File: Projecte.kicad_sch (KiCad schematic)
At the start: 52 parts, among them J1 Conn_motor, J2 Conn_01x04_Pin, K1 A161CS12VDC.64, Q1 IRLZ34N, Q3 IRLZ34N, Q4 IRLZ34N, Q5 IRLZ34N, Q6 IRLZ34N, Q7 IRLZ34N, U1 PIC18F448-IP, U2 LM358, U3 R-786.5-0.5, U4 MCP2551-I-P, U5 AMS1117-3.3, U6 TXB0108PW, U7 LM7805_TO220, U8 MMC5883MA, Y1 Crystal

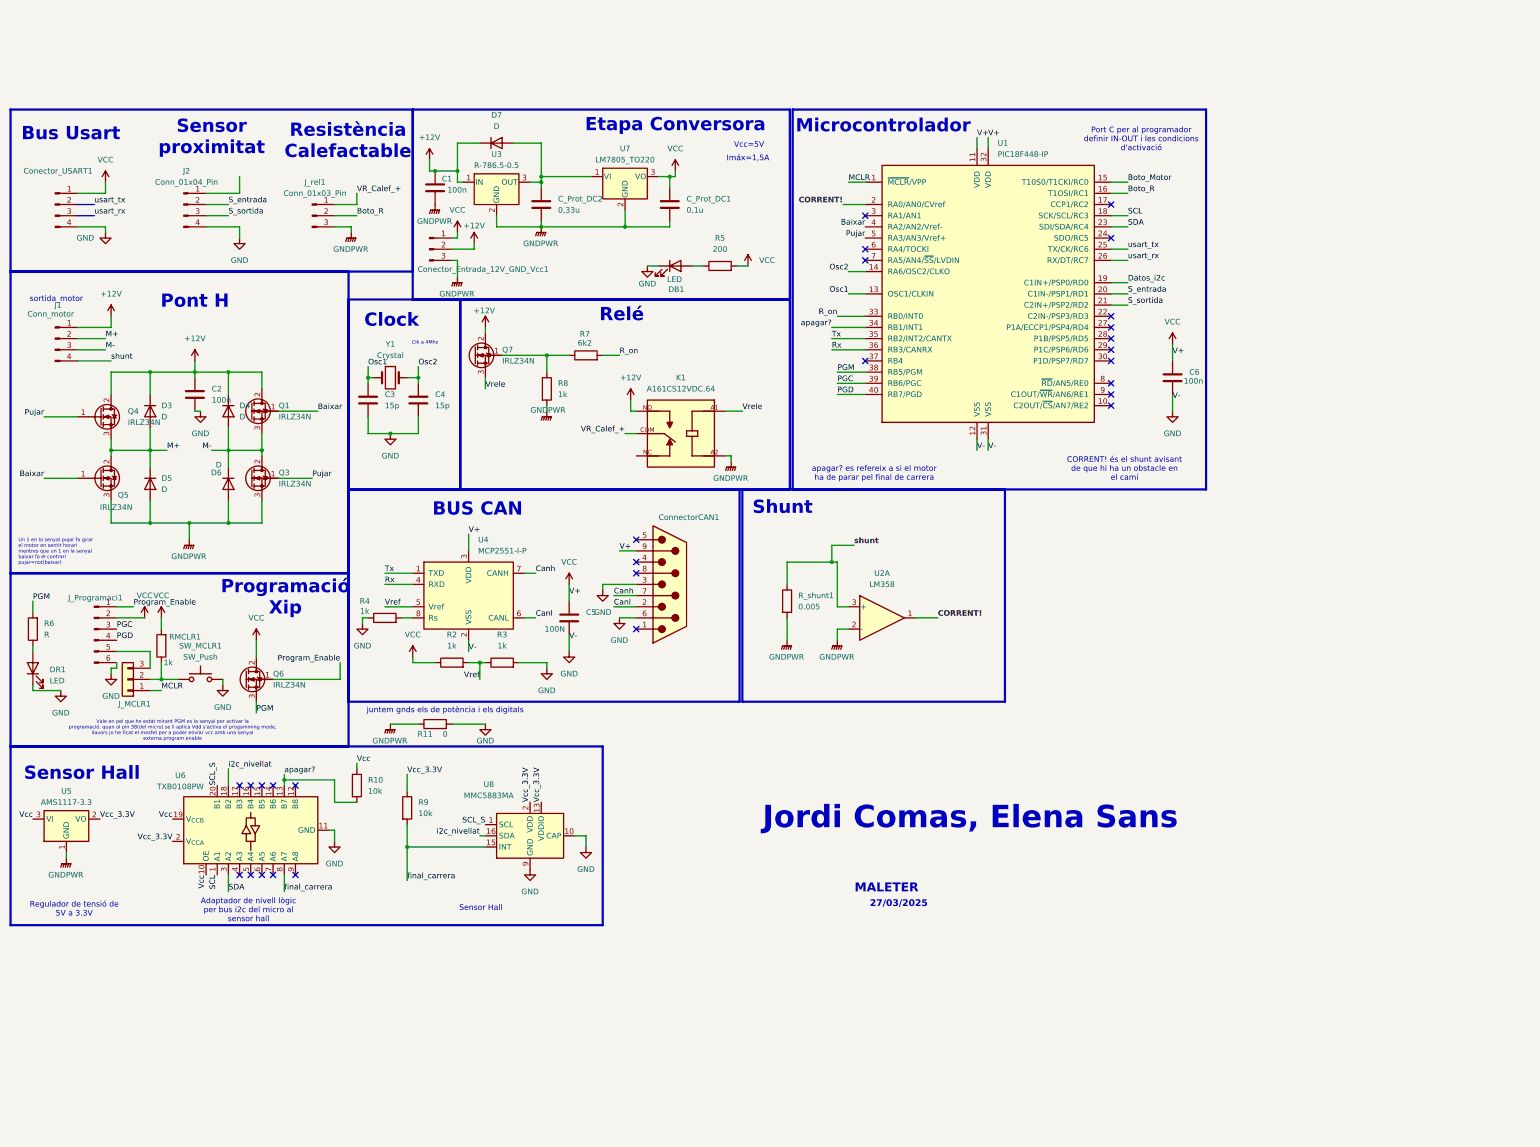
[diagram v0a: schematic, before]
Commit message: Sch_Post_Show
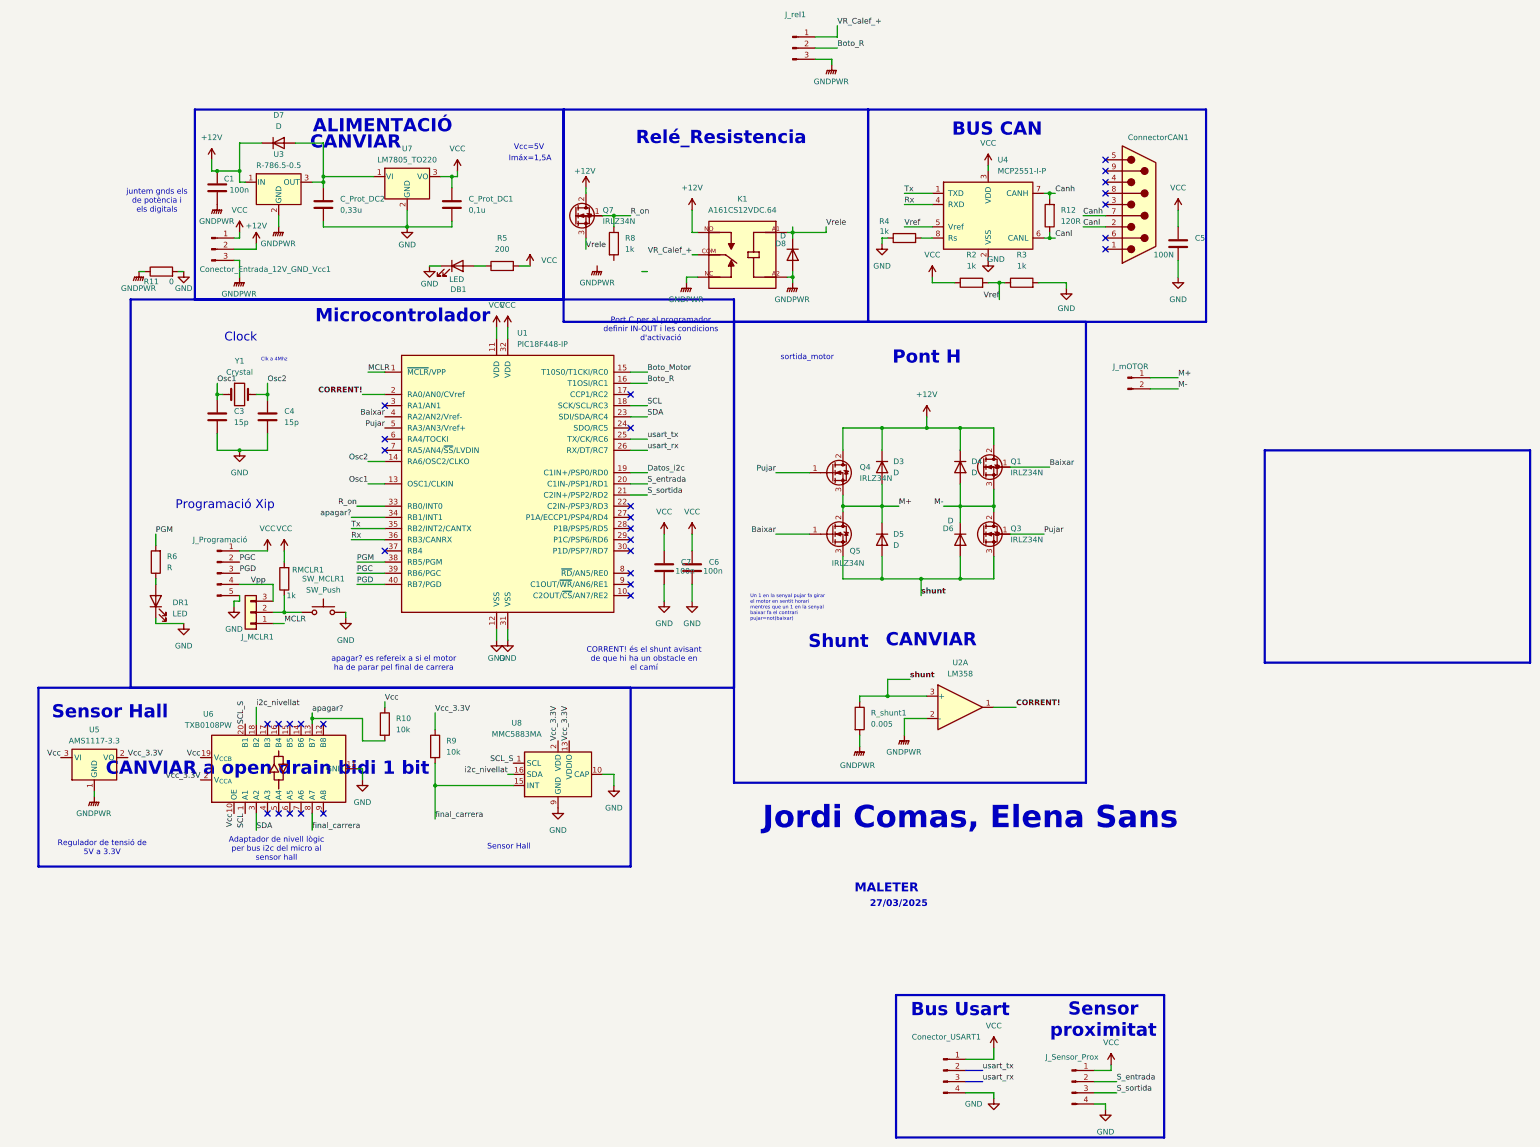
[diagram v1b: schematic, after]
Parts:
- removed C2: 100n, symbol Device:C
- removed J1: Conn_motor, symbol Connector:Conn_01x04_Pin
- removed J_Programaci1: Conn_01x06_Pin, symbol Connector:Conn_01x06_Pin
- removed Q6: IRLZ34N, Package_TO_SOT_THT:TO-220-3_Vertical, symbol Transistor_FET:IRLZ34N
- removed R7: 6k2, symbol Device:R
- added C7: 100n, symbol Device:C
- added D8: D, symbol Device:D
- added J_Programació: Conn_01x05_Pin, symbol Connector:Conn_01x05_Pin
- added J_mOTOR: Conn_01x02_Pin, symbol Connector:Conn_01x02_Pin
- added R12: 120R, symbol Device:R
- renumbered J2 to J_Sensor_Prox
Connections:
- net Canh: now also R12.2
- net Canl: now also R12.1
- net GND: now also C_Prot_DC1.2, C_Prot_DC2.2, U7.2 (GND), C7.2, J_Programació.5 (Pin_5); no longer ConnectorCAN1.3, ConnectorCAN1.6
- net GNDPWR: now also K1.NC, D8.2 (A); no longer C_Prot_DC1.2, C_Prot_DC2.2, D5.2 (A), D6.2 (A), Q3.3 (S), Q5.3 (S), R8.2, U7.2 (GND)
- net M+: now also J_mOTOR.1 (Pin_1)
- net M-: now also J_mOTOR.2 (Pin_2)
- net PGC: now also J_Programació.2 (Pin_2)
- net PGD: now also J_Programació.3 (Pin_3)
- net R_on: now also Q7.1 (G), R8.1
- net VCC: now also J_Sensor_Prox.1 (Pin_1), C7.1, J_Programació.1 (Pin_1); no longer ConnectorCAN1.9
- net Vrele: now also D8.1 (K)
- net shunt: now also D5.2 (A), D6.2 (A), Q3.3 (S), Q5.3 (S)
- net Vpp: now reaches J_MCLR1.3 (Pin_3)
- net Vpp: now also J_Programació.4 (Pin_4)
- no-connect marks 28 -> 31
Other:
- note added: "ALIMENTACIÓ"
- note added: "CANVIAR"
- note added: "CANVIAR a open drain bidi 1 bit"
- note added: "Relé_Resistencia"
- note removed: "Etapa Conversora"
- note removed: "Relé"
- note removed: "Resistència Calefactable"
- note removed: "Vale en pel que he estat mirant PGM es la senyal per activar la programació, quan al pin 38(del micro) se li aplica Vdd s'activa el progamming mode, llavors jo he ficat el mosfet per a poder enviar vcc amb una senyal externa program enable"
- moved on the sheet: C1, C3, C4, C5, C6, C_Prot_DC1, C_Prot_DC2, Conector_Entrada_12V_GND_Vcc1, Conector_USART1, ConnectorCAN1, D3, D4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
